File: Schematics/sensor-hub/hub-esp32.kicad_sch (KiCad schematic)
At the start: 15 parts

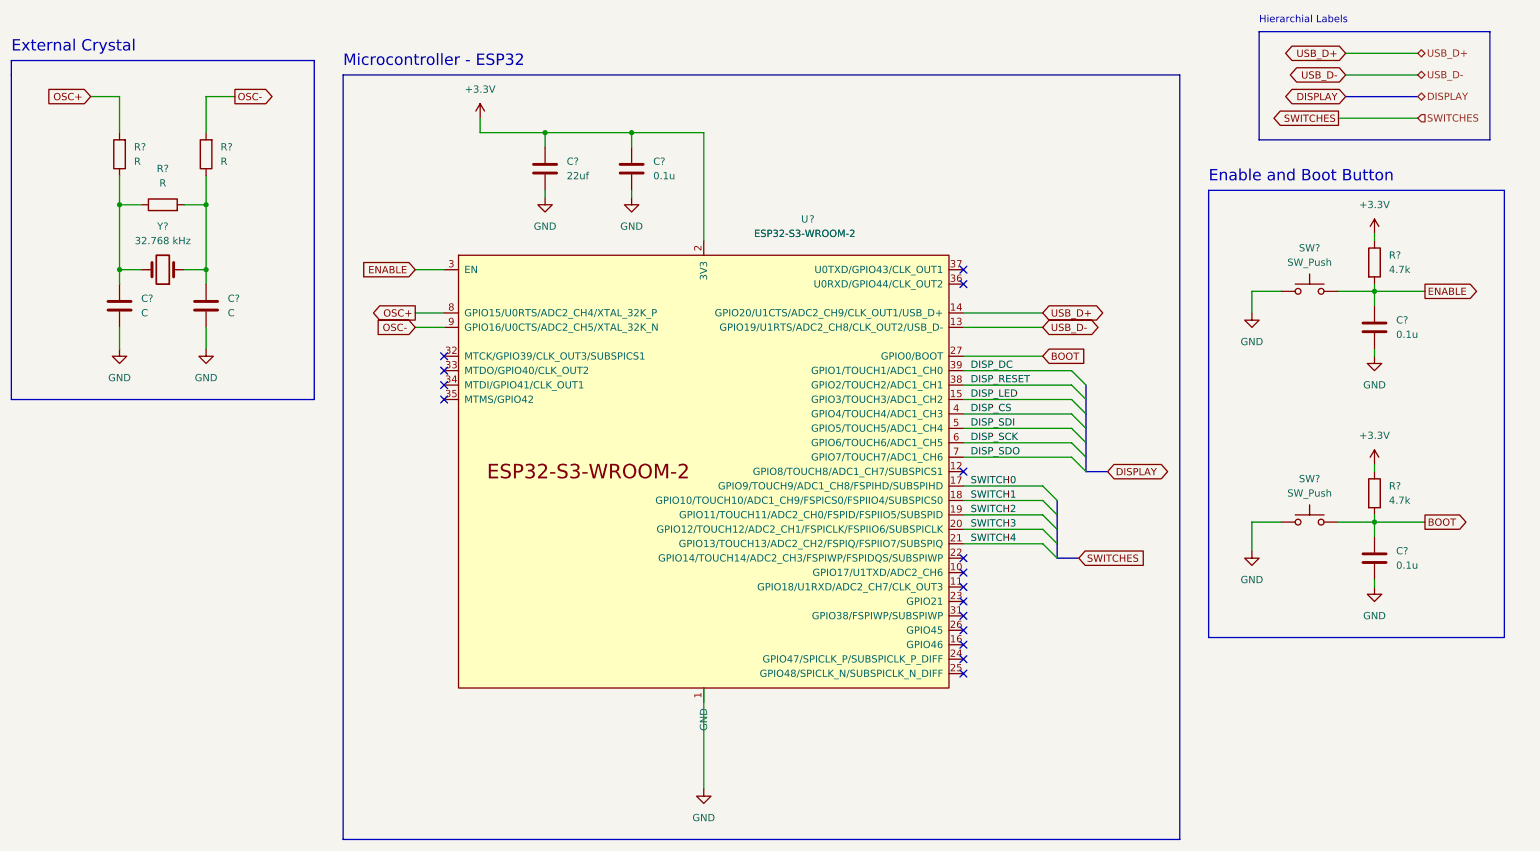
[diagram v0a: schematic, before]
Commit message: schematic and pcb upload
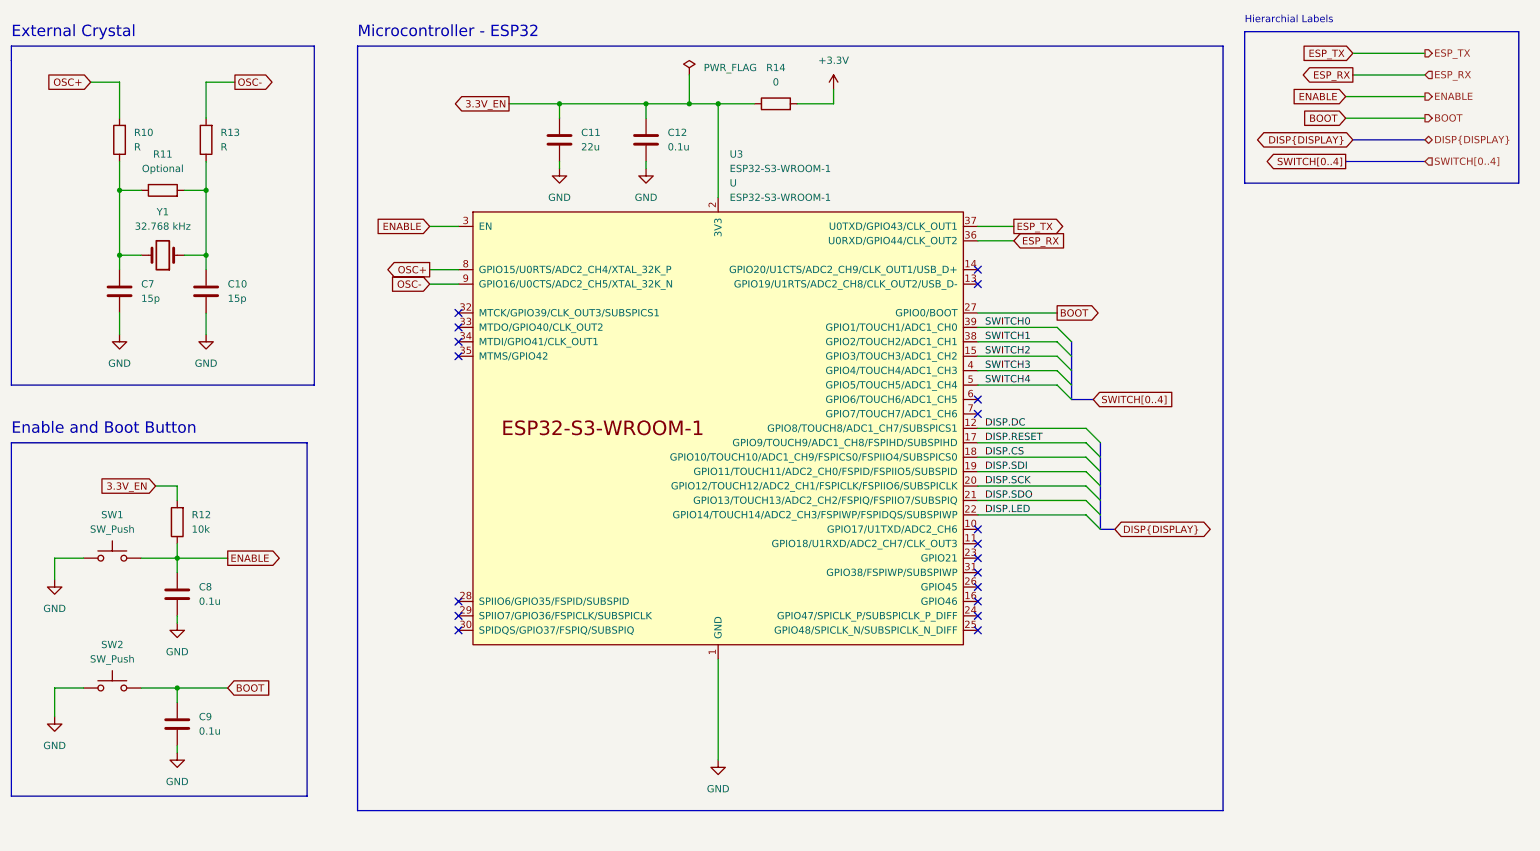
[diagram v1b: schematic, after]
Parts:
- removed ?: ESP32-S3-WROOM-2, symbol Espressif:ESP32-S3-WROOM-2
- removed R? (x2): 4.7k, symbol Device:R
- added R12: 10k, Resistor_SMD:R_0805_2012Metric_Pad1.20x1.40mm_HandSolder, symbol Device:R
- added R14: 0, Resistor_SMD:R_0805_2012Metric_Pad1.20x1.40mm_HandSolder, symbol Device:R
- added U3: ESP32-S3-WROOM-1, Espressif:ESP32-S3-WROOM-1U, symbol Espressif:ESP32-S3-WROOM-1
- C10, C7: renamed from C?; value C -> 15p; footprint (none) -> Capacitor_SMD:C_0805_2012Metric_Pad1.18x1.45mm_HandSolder
- C11: renamed from C?; value 22uf -> 22u; footprint (none) -> Capacitor_SMD:C_0805_2012Metric_Pad1.18x1.45mm_HandSolder
- C12, C8, C9: renamed from C?; footprint (none) -> Capacitor_SMD:C_0805_2012Metric_Pad1.18x1.45mm_HandSolder
- R10, R13: renamed from R?; footprint (none) -> Resistor_SMD:R_0805_2012Metric_Pad1.20x1.40mm_HandSolder
- R11: renamed from R?; value R -> Optional; footprint (none) -> Resistor_SMD:R_0805_2012Metric_Pad1.20x1.40mm_HandSolder
- SW1, SW2: renamed from SW?; footprint (none) -> JLCPCB_Components:Switch_Small
- Y1: renamed from Y?; footprint (none) -> Crystal:Crystal_SMD_3215-2Pin_3.2x1.5mm
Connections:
- net +3V3: now also R14.2; no longer C11.2, C12.2
- net BOOT: now also U3.27 (GPIO0/BOOT)
- net ENABLE: now also R12.1, U3.3 (EN)
- net GND: now also U3.1 (GND), U3.40 (GND), U3.41 (GND)
- net OSC+: now also U3.8 (GPIO15/U0RTS/ADC2_CH4/XTAL_32K_P)
- net OSC-: now also U3.9 (GPIO16/U0CTS/ADC2_CH5/XTAL_32K_N)
- net SWITCH0: now also U3.39 (GPIO1/TOUCH1/ADC1_CH0)
- net SWITCH1: now also U3.38 (GPIO2/TOUCH2/ADC1_CH1)
- net SWITCH2: now also U3.15 (GPIO3/TOUCH3/ADC1_CH2)
- net SWITCH3: now also U3.4 (GPIO4/TOUCH4/ADC1_CH3)
- net SWITCH4: now also U3.5 (GPIO5/TOUCH5/ADC1_CH4)
- new net 3.3V_EN: C11.2, C12.2, R12.2, R14.1, U3.2 (3V3)
- new net DISP.CS: U3.18 (GPIO10/TOUCH10/ADC1_CH9/FSPICS0/FSPIIO4/SUBSPICS0)
- new net DISP.DC: U3.12 (GPIO8/TOUCH8/ADC1_CH7/SUBSPICS1)
- new net DISP.LED: U3.22 (GPIO14/TOUCH14/ADC2_CH3/FSPIWP/FSPIDQS/SUBSPIWP)
- new net DISP.RESET: U3.17 (GPIO9/TOUCH9/ADC1_CH8/FSPIHD/SUBSPIHD)
- new net DISP.SCK: U3.20 (GPIO12/TOUCH12/ADC2_CH1/FSPICLK/FSPIIO6/SUBSPICLK)
- new net DISP.SDI: U3.19 (GPIO11/TOUCH11/ADC2_CH0/FSPID/FSPIIO5/SUBSPID)
- new net DISP.SDO: U3.21 (GPIO13/TOUCH13/ADC2_CH2/FSPIQ/FSPIIO7/SUBSPIQ)
- new net ESP_RX: U3.36 (U0RXD/GPIO44/CLK_OUT2)
- new net ESP_TX: U3.37 (U0TXD/GPIO43/CLK_OUT1)
- no-connect marks 16 -> 19
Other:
- moved on the sheet: C10, C11, C12, C7, C8, C9, R10, R11, R13, SW1, SW2, Y1
